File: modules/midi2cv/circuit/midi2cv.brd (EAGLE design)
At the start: 56.8 x 63.5 mm, 17 parts, among them U1 MICROCHIP_MCP4902-E-PMICROCHI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, U2 MICROCHIP_MCP4902-E-PMICROCHI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, U3 MICROCHIP_MCP4902-E-PMICROCHI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

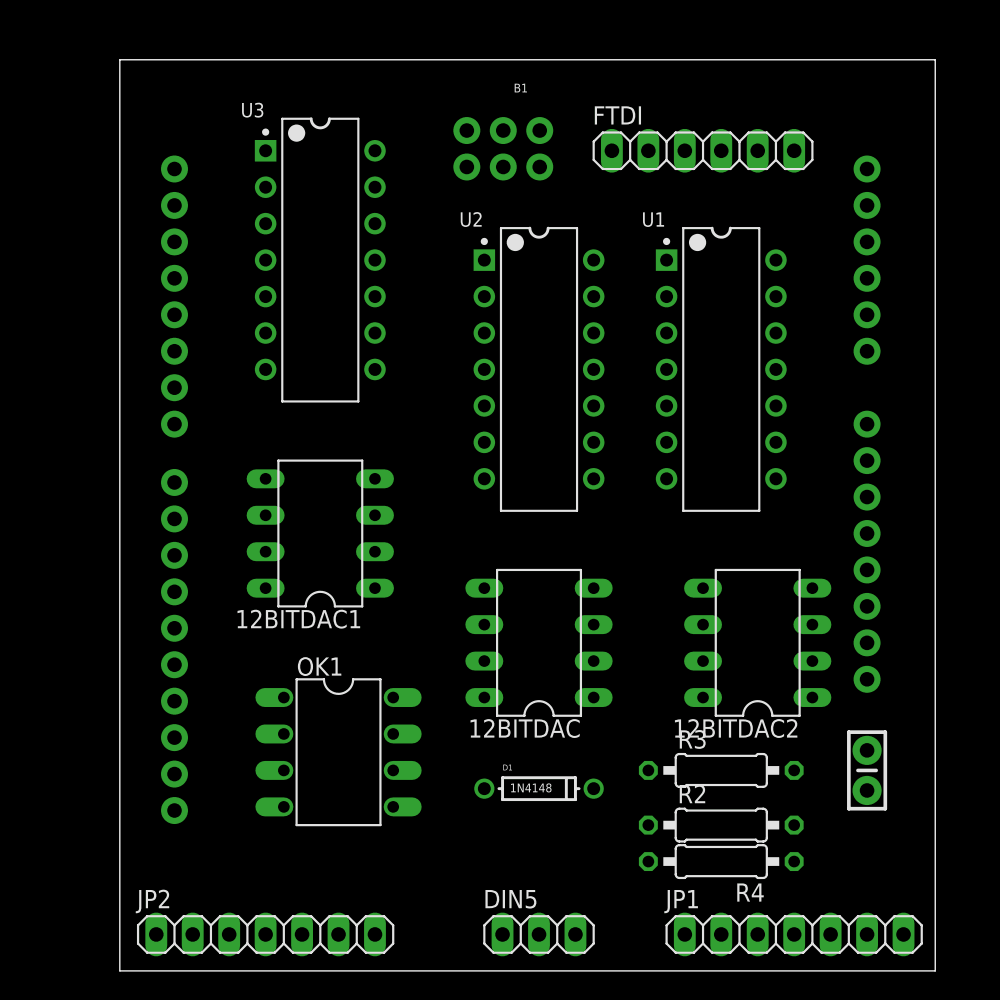
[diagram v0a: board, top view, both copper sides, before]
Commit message: midi2cv
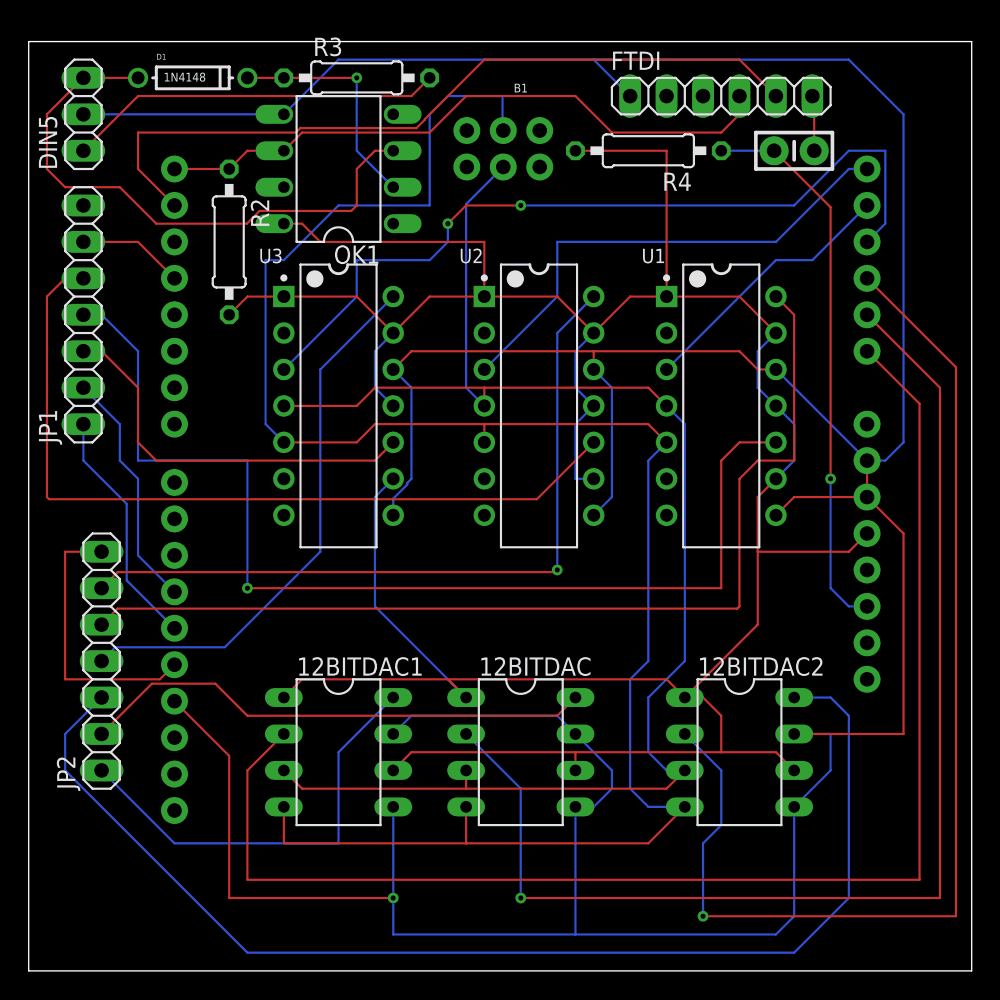
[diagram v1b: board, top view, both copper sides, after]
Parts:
- moved JP1 65.7 mm to (40.6, 45.7), turned to 90 degrees
- moved DIN5 65.4 mm to (40.6, 59.7), turned to 90 degrees
- moved D1 55.1 mm to (48.3, 62.2)
- moved R3 54.5 mm to (59.7, 62.2)
- moved R2 53.2 mm to (50.8, 50.8), turned to 270 degrees
- moved R4 49.8 mm to (80.0, 57.1)
- moved C1 43.5 mm to (90.2, 57.1), turned to 180 degrees
- moved OK1 40.6 mm to (58.4, 55.9), turned to 90 degrees
- moved JP2 22.2 mm to (41.9, 21.6), turned to 90 degrees
- moved 12BITDAC1 15.3 mm to (58.4, 15.2), turned to 270 degrees
- moved U3 10.2 mm to (58.4, 39.4)
- moved 12BITDAC 7.73 mm to (71.1, 15.2), turned to 270 degrees
- moved 12BITDAC2 7.73 mm to (86.4, 15.2), turned to 270 degrees
- moved FTDI 4.02 mm to (85.1, 61.0)
- moved U1 2.54 mm to (85.1, 39.4)
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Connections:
- net +5V: now also U1.9, U2.9, U3.9
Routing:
- net GND: track 0.00 -> 295.8 mm, vias 0 -> 1
- net +5V: track 0.00 -> 221.2 mm
- net MOSI: track 0.00 -> 133.2 mm
- net SCK: track 0.00 -> 106.3 mm
- net CS1: track 0.00 -> 96.4 mm
- net CS2: track 0.00 -> 85.0 mm, vias 0 -> 1
- net PITCH_CV3: track 0.00 -> 84.6 mm
- net CS3: track 0.00 -> 78.9 mm, vias 0 -> 1
- net CC2: track 0.00 -> 75.2 mm, vias 0 -> 1
- net LEVEL2: track 0.00 -> 70.2 mm
- net CS4: track 0.00 -> 57.3 mm, vias 0 -> 2
- net CC3: track 0.00 -> 56.8 mm
- net TX: track 0.00 -> 53.8 mm
- net LEVEL3: track 0.00 -> 52.5 mm, vias 0 -> 1
- net RX: track 0.00 -> 44.3 mm
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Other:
- board size 56.8 x 63.5 mm -> 65.7 x 64.8 mm
